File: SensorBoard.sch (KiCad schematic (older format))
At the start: 10 parts

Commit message: Incorporated STM32F405RGT
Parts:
- added U?: STM32F405RGTx, Package_QFP:LQFP-64_10x10mm_P0.5mm, symbol MCU_ST_STM32F4:STM32F405RGTx
- U?: symbol SensorBoard:MS5607-02BA -> SensorBoard-rescue:MS5607-02BA-SensorBoard
- U?: symbol SensorBoard:BMF055 -> SensorBoard-rescue:BMF055-SensorBoard
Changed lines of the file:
@@
 $EndDescr
 $Comp
-L SensorBoard:MS5607-02BA U?
+L SensorBoard-rescue:MS5607-02BA-SensorBoard U?
 U 1 1 5BFAF6AC
 P 1825 1850
@@
 VDD+3V
 $Comp
-L SensorBoard:BMF055 U?
+L SensorBoard-rescue:BMF055-SensorBoard U?
 U 1 1 5C02E18B
 P 2675 4725
@@
 	1    0    0    -1
 $EndComp
+$Comp
+L MCU_ST_STM32F4:STM32F405RGTx U?
+U 1 1 5C1DE3B9
+P 5550 4950
+F 0 "U?" H 4950 6700 50  0000 L CNN
+F 1 "STM32F405RGTx" H 5950 6700 50  0000 L CNN
+F 2 "Package_QFP:LQFP-64_10x10mm_P0.5mm" H 4950 3250 50  0001 R CNN
+F 3 "http://www.st.com/st-web-ui/static/active/en/resource/technical/document/datasheet/DM00037051.pdf" H 5550 4950 50  0001 C CNN
+	1    5550 4950
+	1    0    0    -1
+$EndComp

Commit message: new board
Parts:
- removed U?: STM32F405RGTx, Package_QFP:LQFP-64_10x10mm_P0.5mm, symbol MCU_ST_STM32F4:STM32F405RGTx
- U?: symbol SensorBoard-rescue:MS5607-02BA-SensorBoard -> SensorBoard:MS5607-02BA
- U?: symbol SensorBoard-rescue:BMF055-SensorBoard -> SensorBoard:BMF055
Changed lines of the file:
@@
 $EndDescr
 $Comp
-L SensorBoard-rescue:MS5607-02BA-SensorBoard U?
+L SensorBoard:MS5607-02BA U?
 U 1 1 5BFAF6AC
 P 1825 1850
@@
 VDD+3V
 $Comp
-L SensorBoard-rescue:BMF055-SensorBoard U?
+L SensorBoard:BMF055 U?
 U 1 1 5C02E18B
 P 2675 4725
@@
 	1    0    0    -1
 $EndComp
-$Comp
-L MCU_ST_STM32F4:STM32F405RGTx U?
-U 1 1 5C1DE3B9
-P 5550 4950
-F 0 "U?" H 4950 6700 50  0000 L CNN
-F 1 "STM32F405RGTx" H 5950 6700 50  0000 L CNN
-F 2 "Package_QFP:LQFP-64_10x10mm_P0.5mm" H 4950 3250 50  0001 R CNN
-F 3 "http://www.st.com/st-web-ui/static/active/en/resource/technical/document/datasheet/DM00037051.pdf" H 5550 4950 50  0001 C CNN
-	1    5550 4950
-	1    0    0    -1
-$EndComp

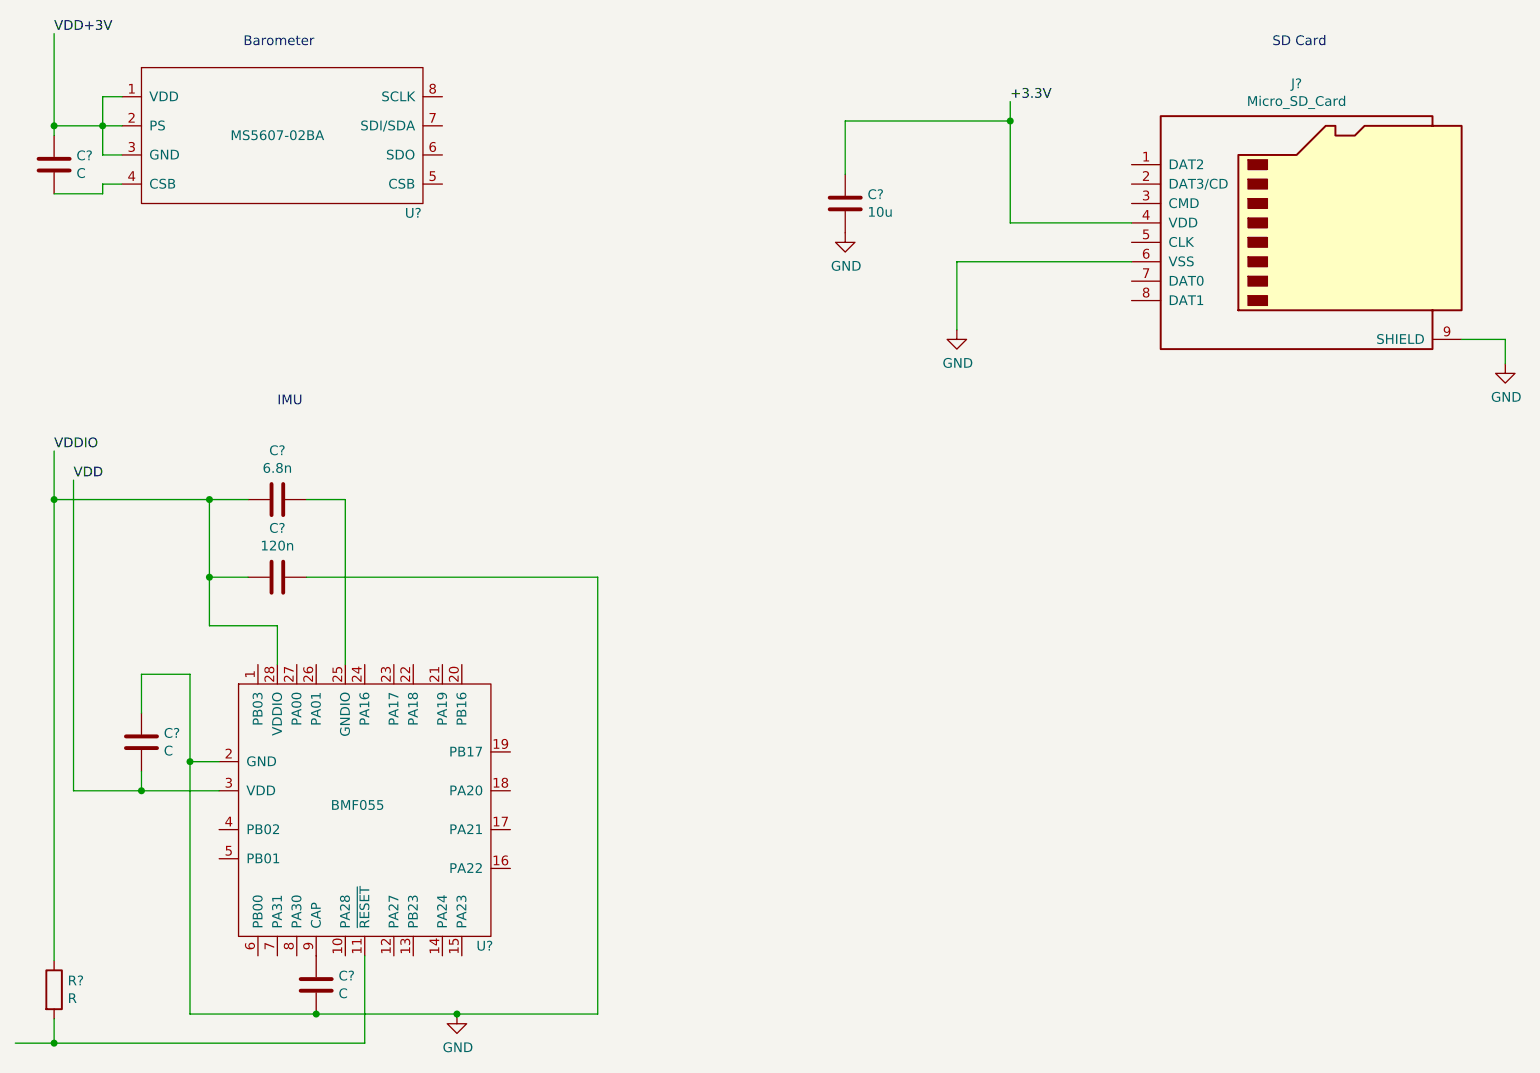
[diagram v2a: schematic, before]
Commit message: Finalized Sensor Board
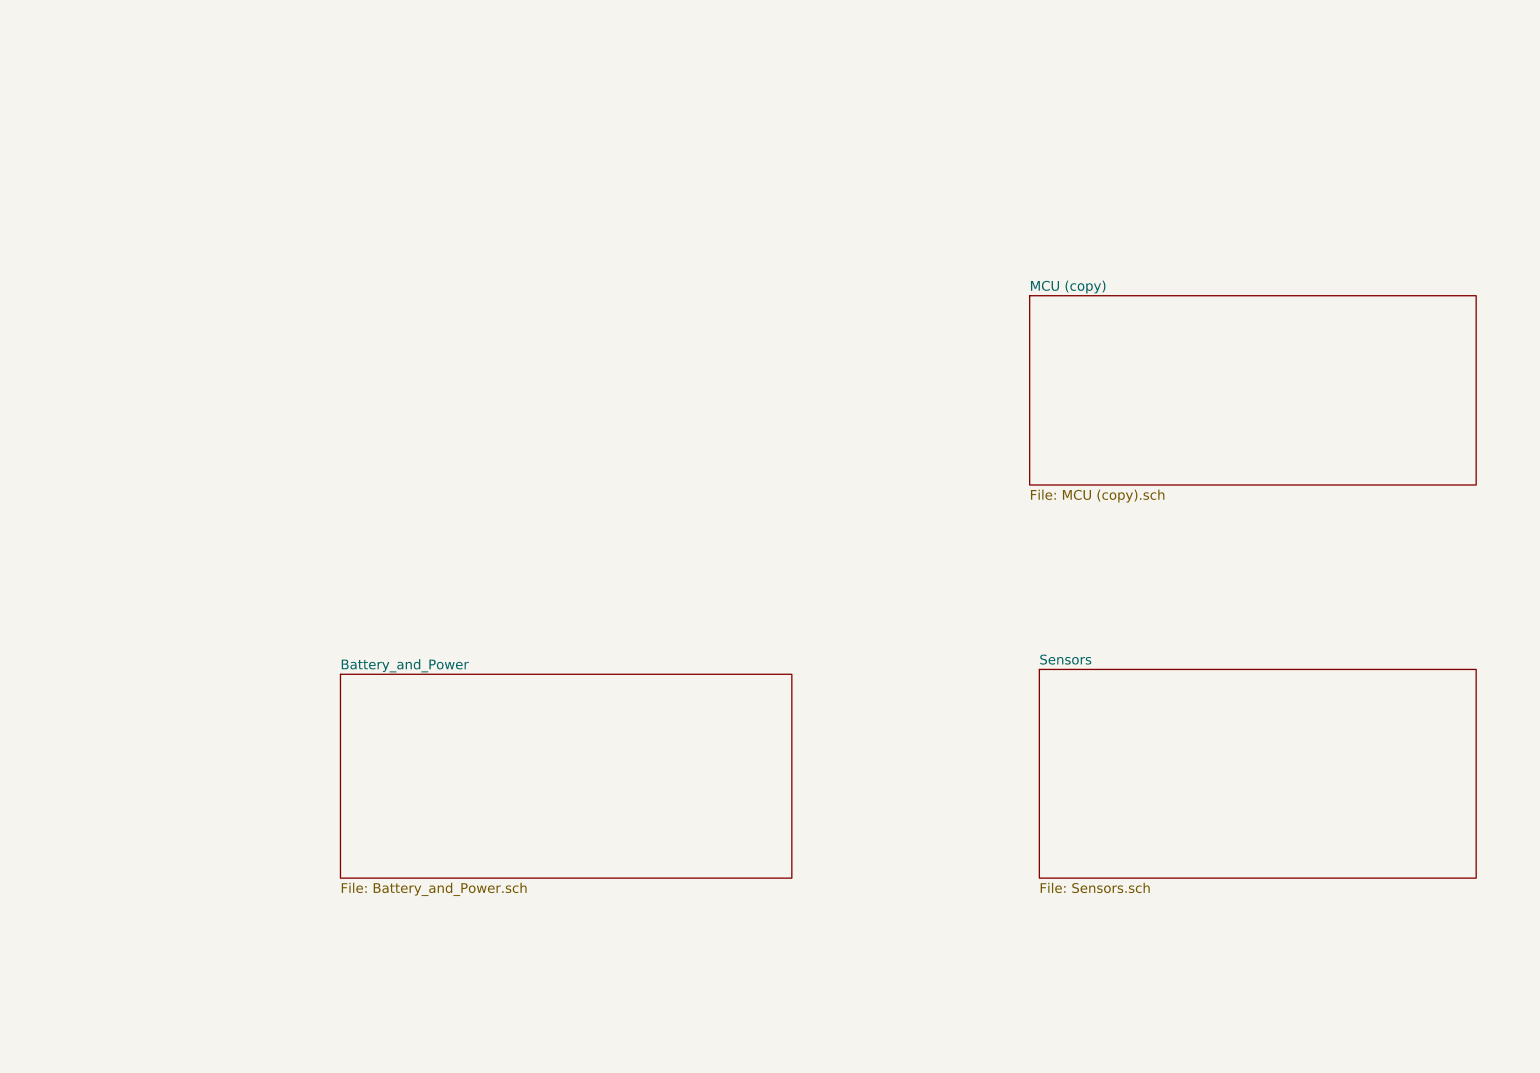
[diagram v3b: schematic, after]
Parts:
- removed C? (x3): C, symbol Device:C
- removed C?: 120n, symbol Device:C
- removed C?: 6.8n, symbol Device:C
- removed C?: 10u, symbol Device:C
- removed J?: Micro_SD_Card, symbol Connector:Micro_SD_Card
- removed R?: R, symbol Device:R
- removed U?: MS5607-02BA, symbol SensorBoard:MS5607-02BA
- removed U?: BMF055, symbol SensorBoard:BMF055
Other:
- note removed: "Barometer"
- note removed: "IMU"
- note removed: "SD Card"
